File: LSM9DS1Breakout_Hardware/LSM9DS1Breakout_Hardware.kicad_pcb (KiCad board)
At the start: 2 copper layers, 8 parts, among them U1 Adafruit_LSM9DS1

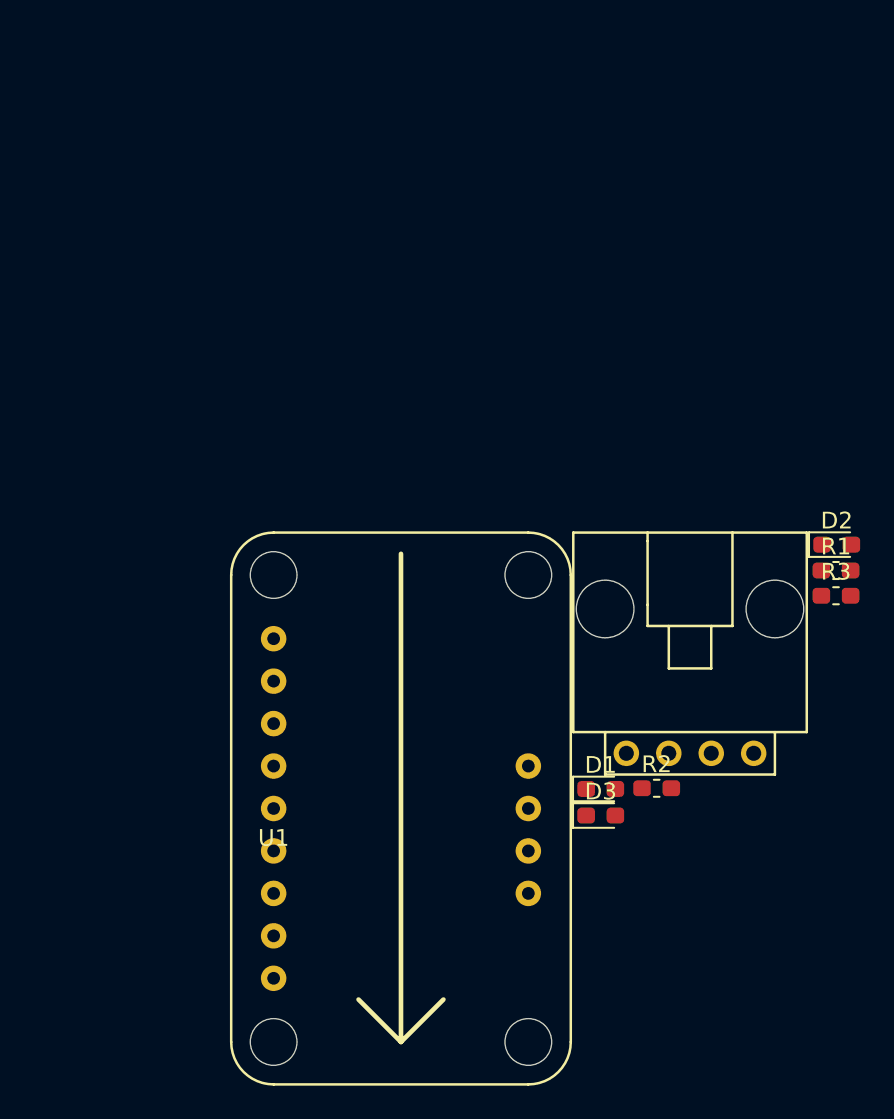
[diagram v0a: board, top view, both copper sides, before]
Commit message: did layout
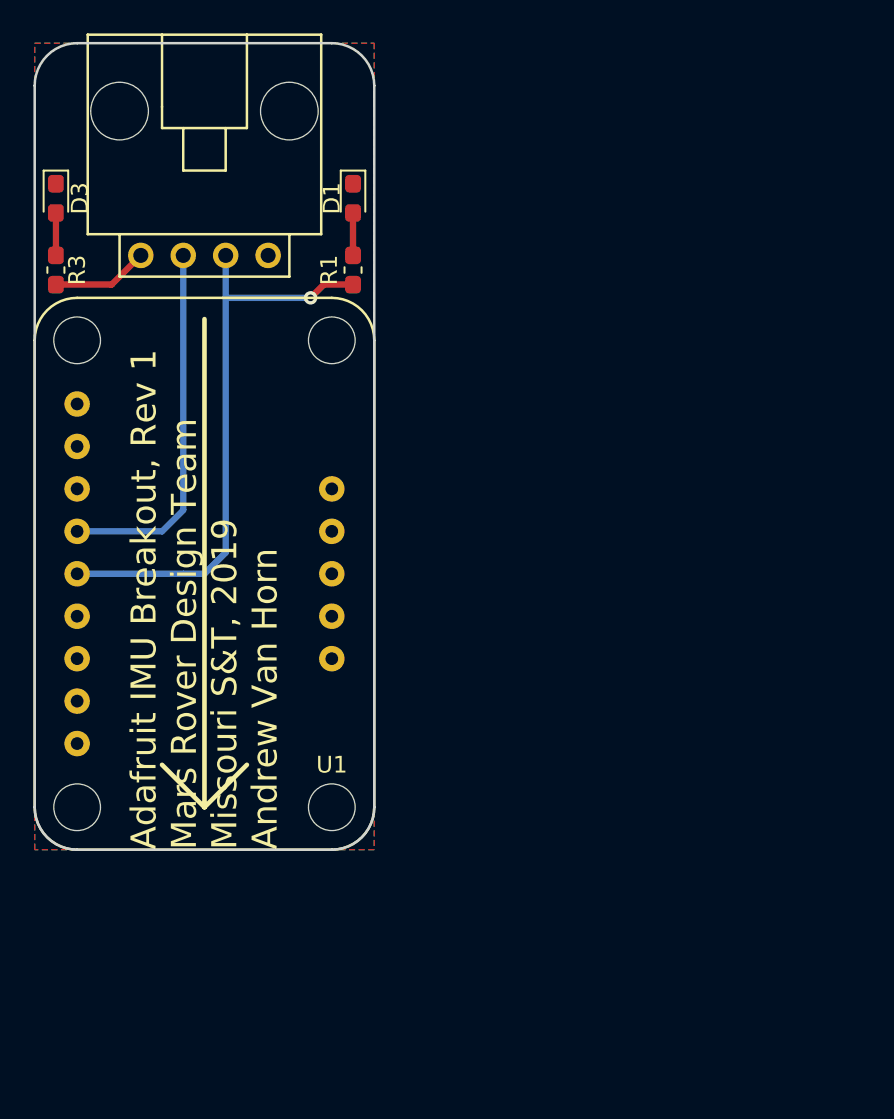
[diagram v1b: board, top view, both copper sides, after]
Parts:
- removed D2: LED, LED_SMD:LED_0603_1608Metric_Pad1.05x0.95mm_HandSolder
- removed R2: 500, Resistor_SMD:R_0603_1608Metric_Pad1.05x0.95mm_HandSolder
- moved R3 50.6 mm to (120.7, 37.7), turned to 90 degrees
- moved D3 49.3 mm to (120.7, 33.4), turned to 270 degrees
- moved Conn1 41.6 mm to (129.5, 36.8)
- moved D1 38.3 mm to (138.4, 33.4), turned to 270 degrees
- moved R1 34.0 mm to (138.4, 37.7), turned to 90 degrees
- moved U1 18.3 mm to (121.9, 55.9)
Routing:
- net SDA: track 0.00 -> 35.1 mm, vias 0 -> 1
- net SCL: track 0.00 -> 22.1 mm
- net +5V: track 0.00 -> 5.80 mm
- net Net-(D3-Pad2): track 0.00 -> 2.54 mm
- net Net-(D1-Pad2): track 0.00 -> 2.54 mm
- added copper zone on B.Cu, net +5V
- added copper zone on F.Cu, net GND
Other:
- board outline added: 20.3 x 48.3 mm
- board text added: "5V"
- board text added: "Adafruit IMU Breakout, Rev 1 Mars Rover Design Team Missouri S&T, 2019 Andrew Van Horn"
- board text added: "GND"
- board text added: "N"
- board text added: "SCL"
- board text added: "SDA"
